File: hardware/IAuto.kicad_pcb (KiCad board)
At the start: 2 copper layers, 56 x 85 mm, 66 parts, among them J1 Barrel_Jack_Switch, J2 4R7uH, J3 4R7uH, J4 M1, J5 M2, J6 Cable_PAD, J7 Cable_PAD, J8 Cable_PAD, J9 Cable_PAD, P1 CONN_02X20, P2 CONN_02X05, Q1 SI4835DDY-T1-GE3, Q2 2N7002, Q3 2N7002, Q4 2N7002, Q5 2N7002, U1 ESP32_NODEMCU, U2 MP1584, U3 MP1584, U4 DRV8833

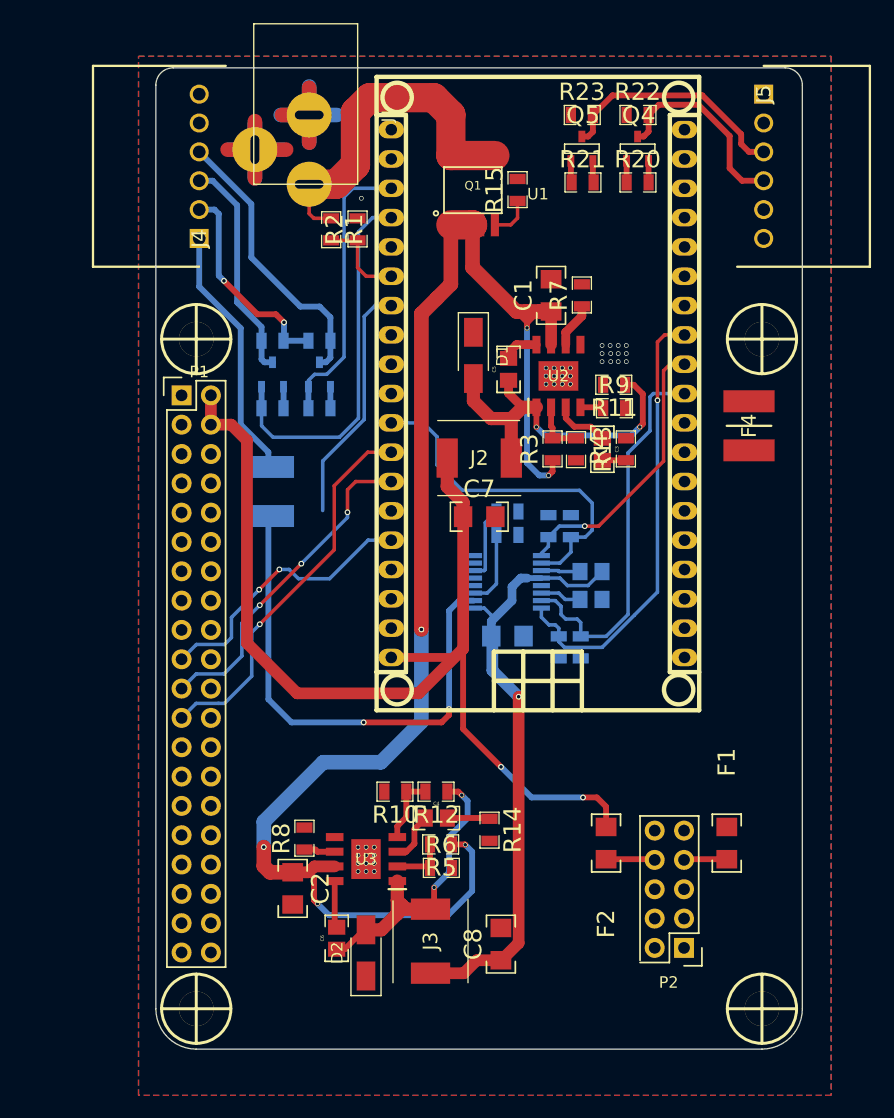
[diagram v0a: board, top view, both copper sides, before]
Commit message: hardware
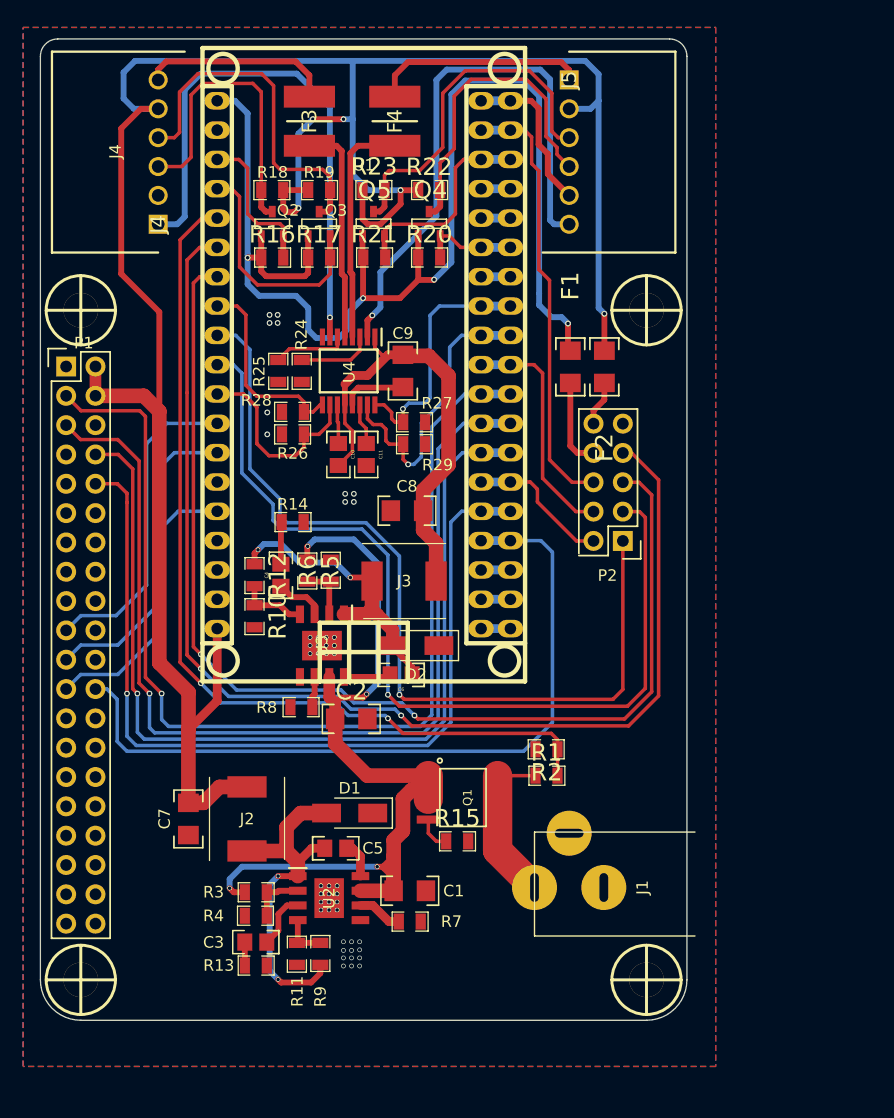
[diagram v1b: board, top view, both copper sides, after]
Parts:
- C10, C11, C9, F3, Q2, Q3, R16, R17, R18, R19, R24, R25, R26, R27, R28, R29, U4: moved to F.Cu
- moved J1 71.6 mm to (170.3, 112.0), turned to 180 degrees
- moved R15 56.7 mm to (157.6, 108.0), turned to 0 degrees
- moved R7 56.3 mm to (153.5, 115.0), turned to 0 degrees
- moved R11 55.5 mm to (145.7, 117.7), turned to 90 degrees
- moved R13 55.0 mm to (140.2, 118.8), turned to 0 degrees
- moved R9 54.7 mm to (143.7, 117.7), turned to 270 degrees
- moved C1 53.0 mm to (153.5, 112.3), turned to 0 degrees
- moved Q1 52.6 mm to (158.1, 104.2), turned to 270 degrees
- moved C3 52.2 mm to (140.2, 116.7), turned to 180 degrees
- moved R1 50.9 mm to (165.3, 102.3), turned to 0 degrees
- moved U2 49.4 mm to (146.5, 112.9), turned to 0 degrees
- moved R4 49.0 mm to (140.2, 114.4), turned to 180 degrees
- moved R2 47.9 mm to (165.3, 100.0), turned to 180 degrees
- moved R3 46.2 mm to (140.2, 112.4), turned to 0 degrees
- moved C5 44.1 mm to (147.1, 108.6), turned to 0 degrees
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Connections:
- net GPIO35 renamed GPIO34
- F1 pad 2: Net-(F1-Pad2) -> +3V3
- F3 pad 1: /Power Part/AOUT1 -> /Power Part/BOUT2
- F4 pad 1: /Power Part/BOUT1 -> /Power Part/AOUT2
- J4 pad 1: Net-(F3-Pad2) -> /Power Part/BOUT1
- J4 pad 2: +5C -> GND
- J4 pad 3: /Power Part/A1 -> /Power Part/B1
- J4 pad 4: /Power Part/B1 -> /Power Part/A1
- J4 pad 5: GND -> +5V
- J4 pad 6: /Power Part/AOUT2 -> Net-(F3-Pad2)
- J5 pad 2: +5C -> +5V
- J5 pad 6: /Power Part/BOUT2 -> /Power Part/AOUT1
- P2 pad 1: /Logical Part/GPIO34 -> /Logical Part/GPIO25
- P2 pad 10: GND -> +5VF
- P2 pad 2: /Logical Part/GPIO5 -> /Logical Part/GPIO0
- P2 pad 3: (no net) -> /Logical Part/GPIO26
- P2 pad 4: (no net) -> /Logical Part/GPIO5
- P2 pad 5: /Logical Part/GPIO0 -> /Logical Part/GPIO32
- P2 pad 6: /Logical Part/GPIO26 -> /Logical Part/GPIO23
- P2 pad 7: /Logical Part/F+3.3V -> /Logical Part/GPIO35
- P2 pad 8: +5VF -> /Logical Part/F+3.3V
- R18 pad 1: +5C -> +5V
- R19 pad 1: +5C -> +5V
- R22 pad 1: +5C -> +5V
- R23 pad 1: +5C -> +5V
- U1 pad 13: /Logical Part/CLK -> /Logical Part/MOSI
- U1 pad 16: /Logical Part/MOSI -> /Logical Part/CLK
- U1 pad 2: Net-(F1-Pad2) -> +3V3
- U1 pad 20: (no net) -> Net-(U1-Pad20)
- U1 pad 21: (no net) -> Net-(U1-Pad21)
- U1 pad 22: (no net) -> Net-(U1-Pad22)
- U1 pad 23: (no net) -> /Logical Part/CS
- U1 pad 24: AO2 -> /Logical Part/RXD
- U1 pad 26: BO2 -> /Logical Part/TXD
- U1 pad 27: /Logical Part/RXD -> /Logical Part/SCL
- U1 pad 28: /Logical Part/TXD -> /Logical Part/SDA
- U1 pad 30: BIN1 -> AIN2
- U1 pad 33: /Logical Part/SDA -> BO2
- U1 pad 34: (no net) -> Net-(U1-Pad34)
- U1 pad 35: (no net) -> Net-(U1-Pad35)
- U1 pad 36: /Logical Part/SCL -> AO2
- U1 pad 37: (no net) -> /Logical Part/GPIO23
- U1 pad 7: /Logical Part/GPIO34 -> /Logical Part/GPIO35
- U1 pad 8: /Logical Part/CS -> /Logical Part/GPIO32
- U1 pad 9: AIN2 -> BIN1
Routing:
- net /Logical Part/GPIO35: track 0.00 -> 104.5 mm, vias 0 -> 2
- net +5V: track 101.8 -> 204.5 mm, vias 2 -> 5
- net +3V3: track 7.48 -> 110.0 mm, vias 0 -> 4
- net /Logical Part/GPIO32: track 0.00 -> 97.1 mm, vias 0 -> 2
- net /Logical Part/SDA: track 0.00 -> 91.4 mm, vias 0 -> 1
- net /Logical Part/SCL: track 0.00 -> 87.3 mm, vias 0 -> 1
- net /Logical Part/TXD: track 0.00 -> 82.2 mm, vias 0 -> 1
- net /Logical Part/GPIO26: track 0.00 -> 79.9 mm, vias 0 -> 1
- net /Logical Part/RXD: track 0.00 -> 76.2 mm, vias 0 -> 1
- net /Logical Part/GPIO25: track 0.00 -> 75.4 mm, vias 0 -> 1
- net GPIO34: track 7.88 -> 79.2 mm, vias 0 -> 2
- net /Power Part/OUT_BAT: track 131.5 -> 74.0 mm, vias 6 -> 4
- net /Power Part/BOUT1: track 0.00 -> 47.9 mm, vias 0 -> 1
- net /Logical Part/CS: track 21.0 -> 66.3 mm
- net /Logical Part/GPIO23: track 0.00 -> 37.8 mm
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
